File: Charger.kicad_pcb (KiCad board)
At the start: 2 copper layers, 94.2 x 44.5 mm, 42 parts, among them J1 Input, J2 USB1, J3 USB2, Q1 BSC42DN25NS3, T1 760875131, U1 LT1085-5.0, U2 TPS2546, U3 LT3798MPMSETRPBF, U4 RTE0016C

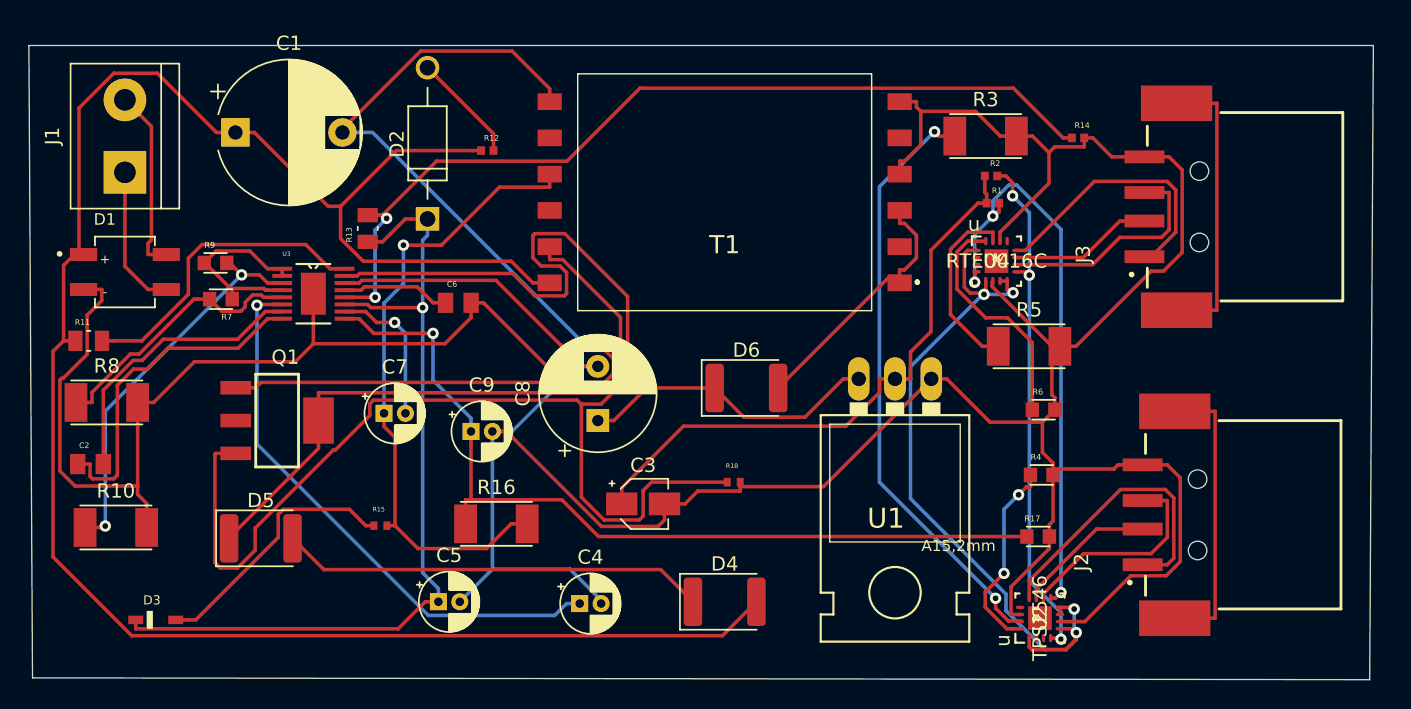
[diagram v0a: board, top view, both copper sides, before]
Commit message: compact
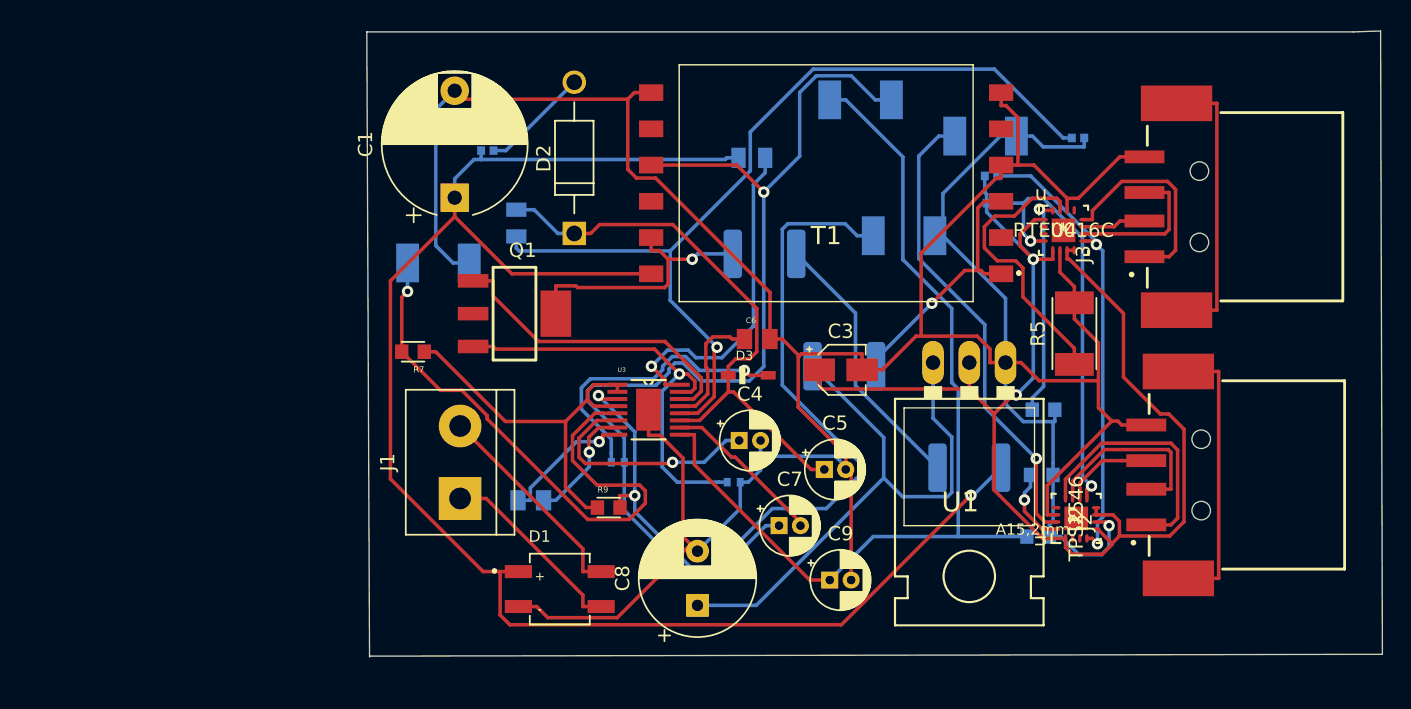
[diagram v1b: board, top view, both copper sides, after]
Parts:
- C2, D4, D5, D6, R1, R10, R11, R12, R13, R14, R15, R16, R17, R18, R2, R3, R4, R6, R8: moved to B.Cu
- moved R10 58.9 mm to (99.3, 43.8)
- moved R11 48.2 mm to (88.6, 38.4)
- moved D3 44.9 mm to (88.4, 53.6)
- moved D5 40.5 mm to (89.5, 45.1)
- moved R16 39.2 mm to (96.3, 34.3)
- moved D1 37.7 mm to (75.2, 68.6)
- moved J1 32.8 mm to (68.2, 62.2)
- moved R9 32.5 mm to (78.6, 62.9)
- moved C2 31.0 mm to (73.2, 62.4)
- moved C7 28.8 mm to (90.6, 64.1)
- moved C5 28.6 mm to (93.7, 60.2)
- moved C9 27.2 mm to (94.1, 67.9)
- moved R8 25.2 mm to (66.7, 45.7)
- moved U3 24.9 mm to (81.4, 56.0)
- moved C6 21.1 mm to (89.0, 51.1)
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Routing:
- net Net-(Q1-Pad3): track 101.2 -> 30.2 mm, vias 0 -> 1
- net gnd: track 300.6 -> 246.2 mm, vias 0 -> 1
- net Net-(R10-Pad1): track 27.5 -> 58.9 mm
- net dcm: track 44.6 -> 74.3 mm
- net Net-(D5-Pad1): track 46.1 -> 18.8 mm, vias 0 -> 1
- net Net-(Q1-Pad1): track 49.2 -> 22.1 mm
- net Net-(C1-Pad1): track 139.0 -> 114.1 mm, vias 0 -> 1
- net Net-(C4-Pad1): track 39.5 -> 16.6 mm
- net Net-(R7-Pad2): track 18.9 -> 41.3 mm, vias 0 -> 1
- net Net-(C8-Pad1): track 21.2 -> 41.7 mm
- net VinL: track 60.5 -> 40.7 mm, vias 1 -> 0
- net Net-(C2-Pad1): track 23.6 -> 9.52 mm, vias 0 -> 1
- net Net-(R7-Pad1): track 13.8 -> 27.2 mm
- net Net-(C2-Pad2): track 20.0 -> 8.55 mm, vias 0 -> 1
- net Stat1: track 41.0 -> 29.6 mm, vias 3 -> 2
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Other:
- board size 94.2 x 44.5 mm -> 71.2 x 43.9 mm
